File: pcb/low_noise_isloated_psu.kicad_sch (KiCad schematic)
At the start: 35 parts, among them Q2 BSS84, U1 LT3094, U13 TDR 3-0523SM, U2 LT3045, U3 LT1763CS8-5

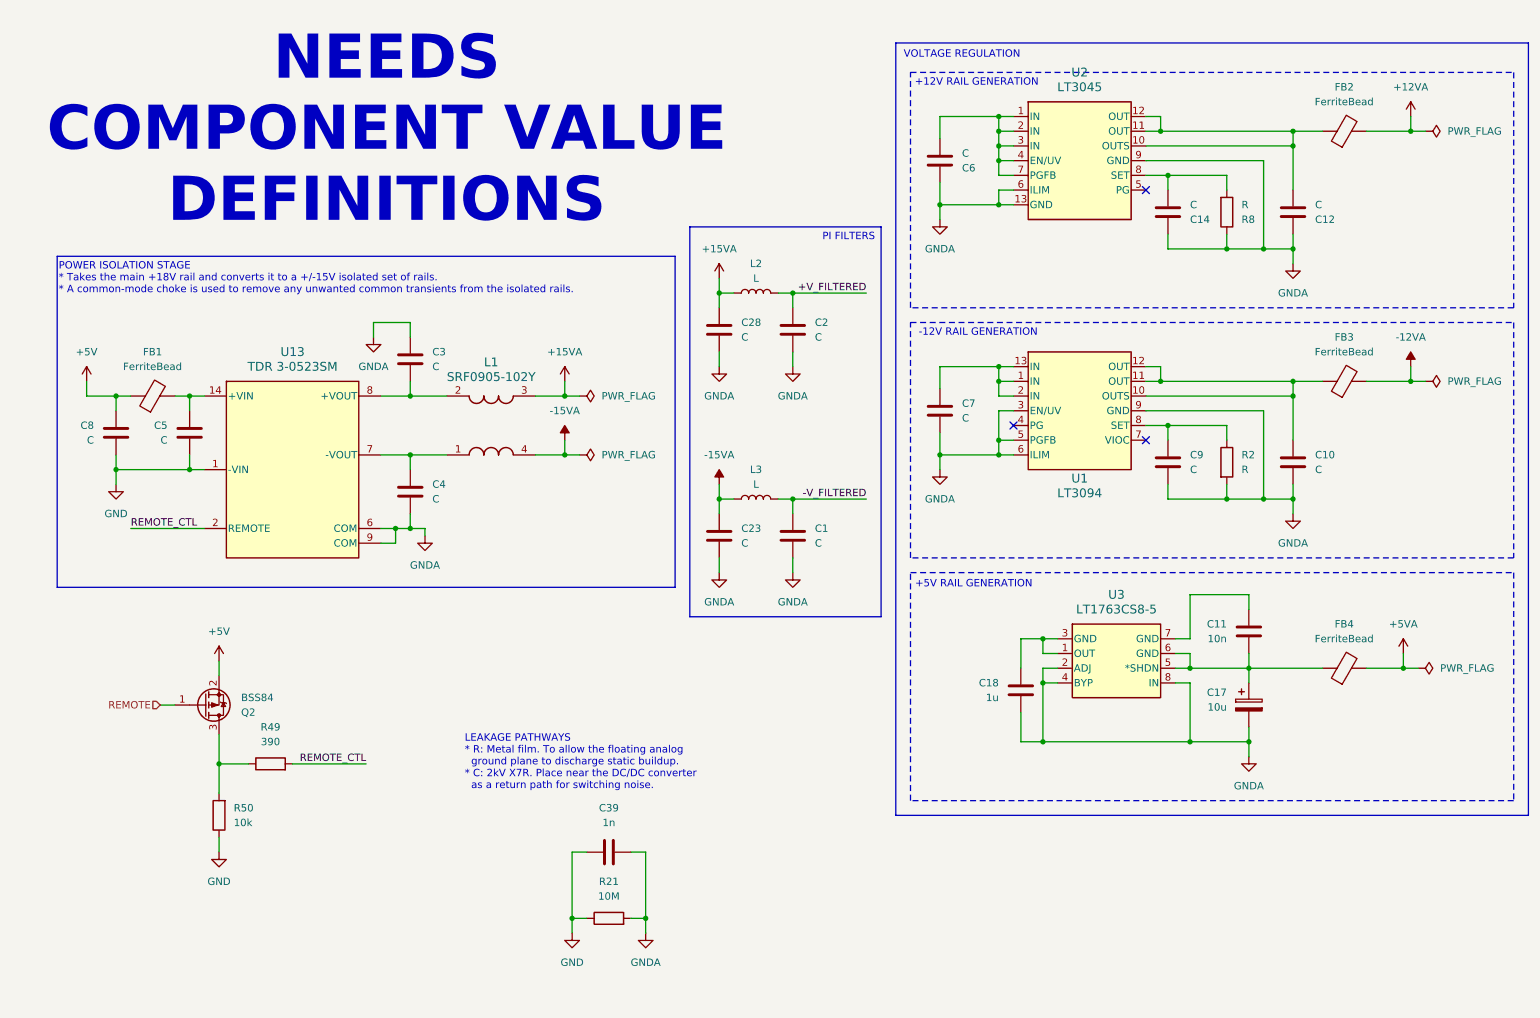
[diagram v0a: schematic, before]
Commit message: chore: many changes checkpoint
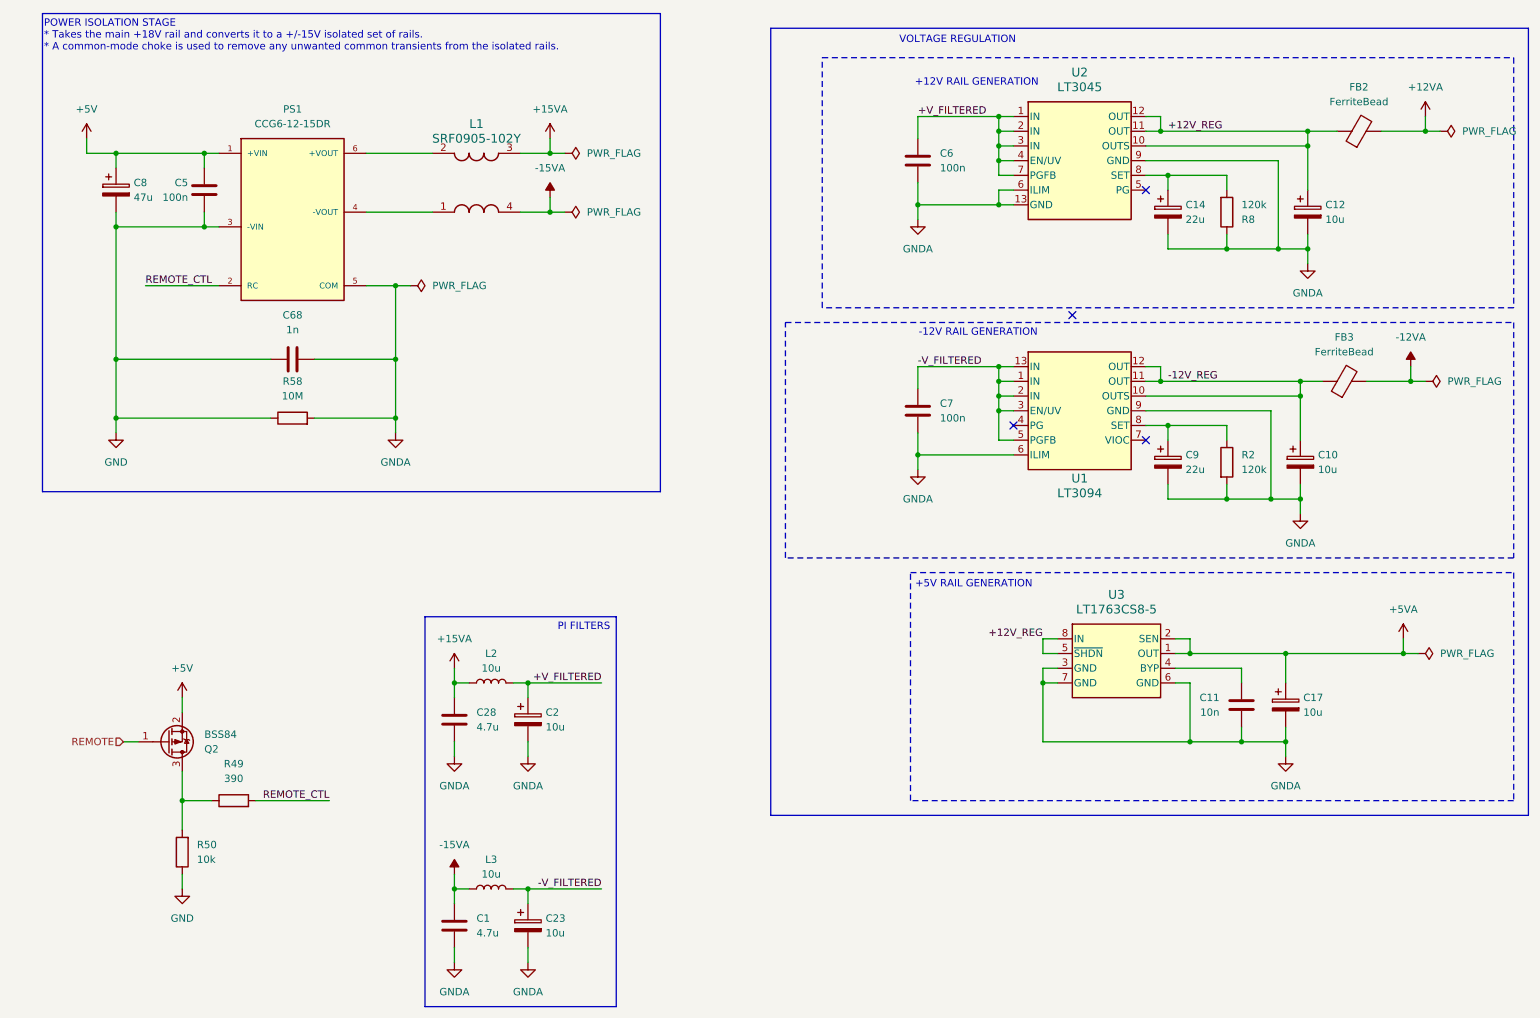
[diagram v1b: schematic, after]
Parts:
- removed C10, C12, C14, C2, C23, C3, C4, C8, C9: C, symbol Device:C
- removed C18: 1u, symbol Device:C
- removed C39: 1n, symbol Device:C
- removed FB1, FB4: FerriteBead, symbol Device:FerriteBead
- removed R21: 10M, symbol Device:R
- removed U13: TDR 3-0523SM, TDR 3SM DUAL_TRP, symbol project_library:TDR_3-0523SM
- added C10, C12, C2, C23: 10u, Capacitor_Tantalum_SMD:CP_EIA-3528-21_Kemet-B, symbol Device:C_Polarized
- added C14, C9: 22u, Capacitor_Tantalum_SMD:CP_EIA-3528-21_Kemet-B, symbol Device:C_Polarized
- added C68: 1n, Capacitor_SMD:C_1812_4532Metric, symbol Device:C
- added C8: 47u, Capacitor_Tantalum_SMD:CP_EIA-3528-21_Kemet-B, symbol Device:C_Polarized
- added PS1: CCG6-12-15DR, project_library:CONV_CCG6-12-15DR, symbol project_library:CCG6-12-15DR
- added R58: 10M, Resistor_SMD:R_1812_4532Metric, symbol Device:R
- C1, C28: value C -> 4.7u; footprint (none) -> Capacitor_SMD:C_0805_2012Metric
- C11: footprint (none) -> Capacitor_SMD:C_0603_1608Metric
- C17: footprint (none) -> Capacitor_Tantalum_SMD:CP_EIA-3528-21_Kemet-B
- C5, C6, C7: value C -> 100n; footprint (none) -> Capacitor_SMD:C_0603_1608Metric
- FB2, FB3: footprint (none) -> Inductor_SMD:L_0603_1608Metric
- L1: footprint SMT_905-102Y_BRN -> project_library:SMT_905-102Y_BRN
- L2, L3: value L -> 10u; footprint (none) -> Inductor_SMD:L_6.3x6.3_H3
- R2, R8: value R -> 120k; footprint (none) -> Resistor_SMD:R_0603_1608Metric
- R49, R50: footprint (none) -> Resistor_SMD:R_0201_0603Metric
- U1: footprint 05-08-1666_ADI -> Package_SO:MSOP-12-1EP_3x4.039mm_P0.65mm_EP1.651x2.845mm
- U2: footprint MSOP12_MSE_ADI -> Package_SO:MSOP-12-1EP_3x4.039mm_P0.65mm_EP1.651x2.845mm
- U3: footprint SO-8_S_LIT -> Package_SO:SOIC-8_3.9x4.9mm_P1.27mm
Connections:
- net +5V: now also C5.1, C8.1, PS1.1 (+VIN)
- net +5VA: now also C17.1, U3.1 (OUT), U3.2 (SEN)
- net +V_FILTERED: now also C6.1, U2.1 (IN), U2.2 (IN), U2.3 (IN), U2.4 (EN/UV), U2.7 (PGFB), C2.1
- net -15VA: now also C1.1
- net -V_FILTERED: now also C7.1, U1.1 (IN), U1.13 (IN), U1.2 (IN), U1.3 (EN/UV), U1.5 (PGFB), C23.1; no longer C1.1
- net GND: now also C68.1, C8.2, PS1.3 (-VIN), R58.1
- net GNDA: now also C11.2, C6.2, U3.3 (GND), U3.6 (GND), U3.7 (GND), C10.2, C12.2, C14.2, C2.2, C23.2, C68.2, C9.2, PS1.5 (COM), R58.2; no longer C6.1, U1.3 (EN/UV), U1.5 (PGFB), U3.2 (ADJ), U3.4 (BYP), U3.8 (IN)
- net REMOTE_CTL: now also PS1.2 (RC)
- net +12V_REG: now reaches FB2.1, U2.10 (OUTS), U2.11 (OUT), U2.12 (OUT)
- net +12V_REG: now also U3.5 (~{SHDN}), U3.8 (IN), C12.1
- net at R2.1, U1.8 (SET): now also C9.1
- net at L1.1: now also PS1.4 (-VOUT)
- net at L1.2: now also PS1.6 (+VOUT)
- net at C11.1: now also U3.4 (BYP); no longer U3.7 (GND)
- net at R8.2, U2.8 (SET): now also C14.1
- net -12V_REG: now reaches FB3.1, U1.10 (OUTS), U1.11 (OUT), U1.12 (OUT)
- net -12V_REG: now also C10.1
- no-connect marks 3 -> 4
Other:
- note removed: "LEAKAGE PATHWAYS * R: Metal film. To allow the floating analog ground plane to discharge static buildup. * C: 2kV X7R. Place near the DC/DC converter as a return path for switching noise."
- note removed: "NEEDS COMPONENT VALUE DEFINITIONS"
- moved on the sheet: C11, C5, L2, Q2, R49, R50
